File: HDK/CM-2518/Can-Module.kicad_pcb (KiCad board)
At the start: 2 copper layers, 34.5 x 14.2 mm, 12 parts, among them J101 Can Connect, J102 Can Connect, J103 Can Termination, U101 SN65HVD230, U102 MCP2518FD, Y101 40MHz

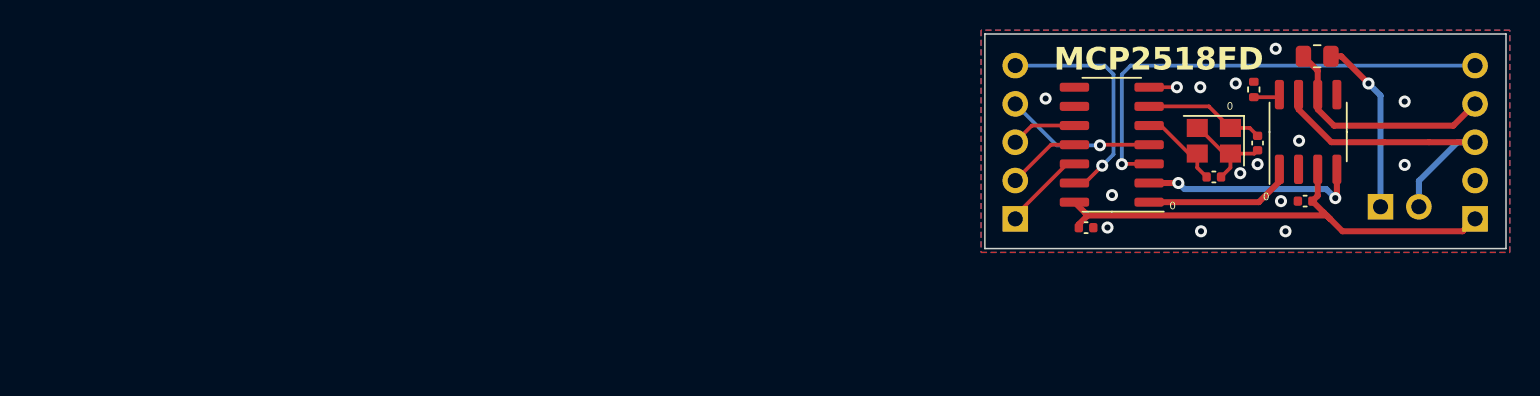
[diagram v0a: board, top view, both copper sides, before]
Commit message: updated can-module
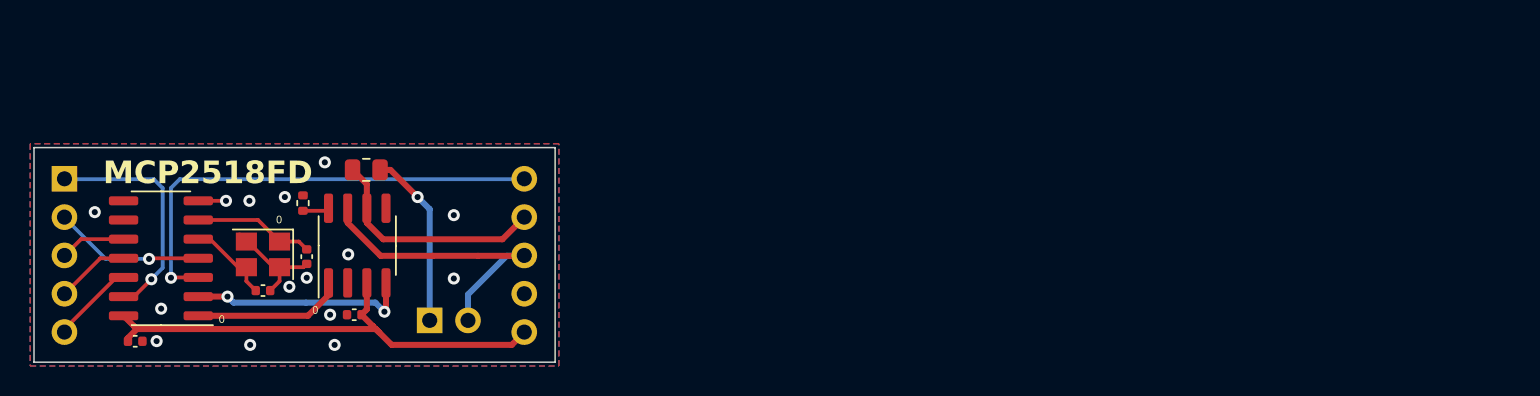
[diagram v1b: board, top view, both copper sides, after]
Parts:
- removed J102: Can Connect, Connector_PinHeader_2.54mm:PinHeader_1x05_P2.54mm_Vertical
- J101: value Can Connect -> MCP251X; footprint Connector_PinHeader_2.54mm:PinHeader_1x05_P2.54mm_Vertical -> NVF-Kicad:Can-Module-CM251X; moved to F.Cu
- moved C102 63.5 mm to (104.0, 103.9)
- moved C103 63.5 mm to (100.8, 100.1)
- moved J103 63.5 mm to (109.0, 104.3)
- moved R101 63.5 mm to (100.6, 96.5)
- moved R102 63.5 mm to (104.8, 94.3)
- moved U101 63.5 mm to (91.2, 100.2)
- moved C101 63.5 mm to (89.5, 105.7)
- moved C104 63.5 mm to (97.9, 102.3)
- moved U102 63.5 mm to (104.2, 99.3)
- moved Y101 63.5 mm to (97.9, 99.9)
- moved J101 47.8 mm to (100.0, 100.0)
- renumbered U102 to U101, U101 to U102
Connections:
- J101 pad 1: /SPI_MISO -> /~{CS}
- J101 pad 2: /SPI_MOSI -> /CAN_IRQ
- J101 pad 4: /CAN_IRQ -> /SPI_MOSI
- J101 pad 5: /~{CS} -> /SPI_MISO
- R102 pad 1: Net-(J103-Pin_1) -> Net-(J102-Pin_1)
